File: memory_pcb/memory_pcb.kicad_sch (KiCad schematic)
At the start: 48 parts, among them J1 Conn_01x10, P1 AFC01-S10FCC-00, U1 AP3602AKTR-G1 SETUPUP, U10 DMG3415U, U11 SS54_C22452, U12 TYPE-C-31-M-12, U2 ESP32-S3-WROOM-1(N16R8), U4 TS-1088-AR02016, U5 TS-1088-AR02016, U6 MAX17048G+T10 FUEL GAUGE, U7 MCP73831T-2ACI/OT Charger, U8 S2B-PH-SM4-TB(LF)(SN)JST-PH C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, U9 AP2112K-3_3TRG1 Regulator

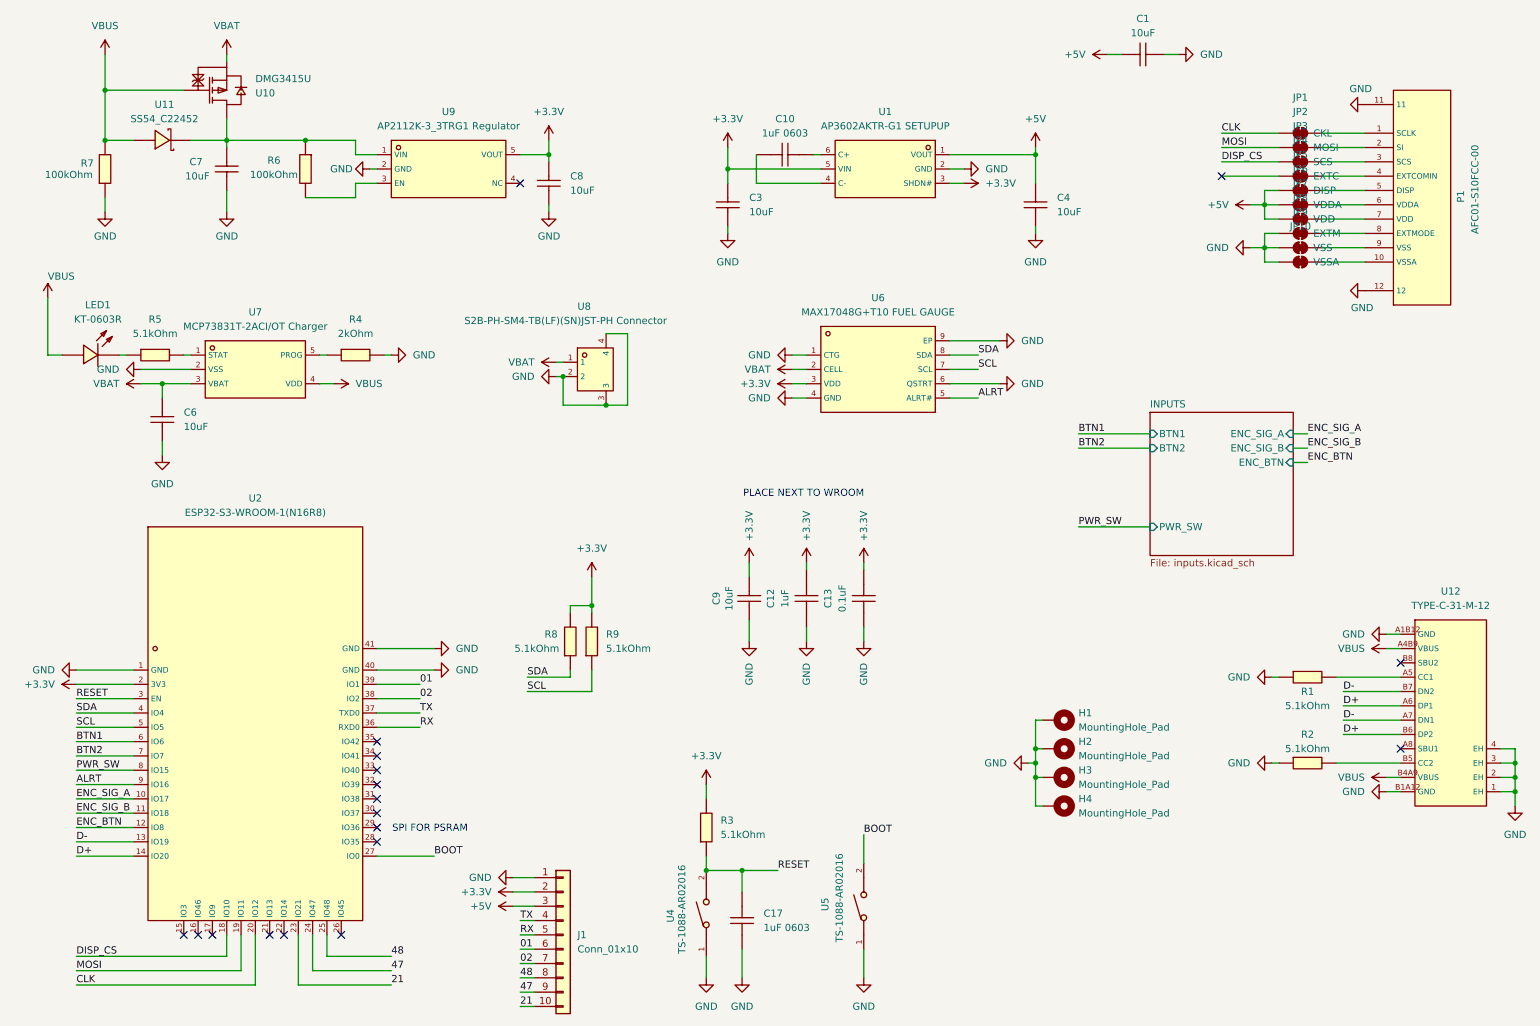
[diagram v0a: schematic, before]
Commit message: looks rdy
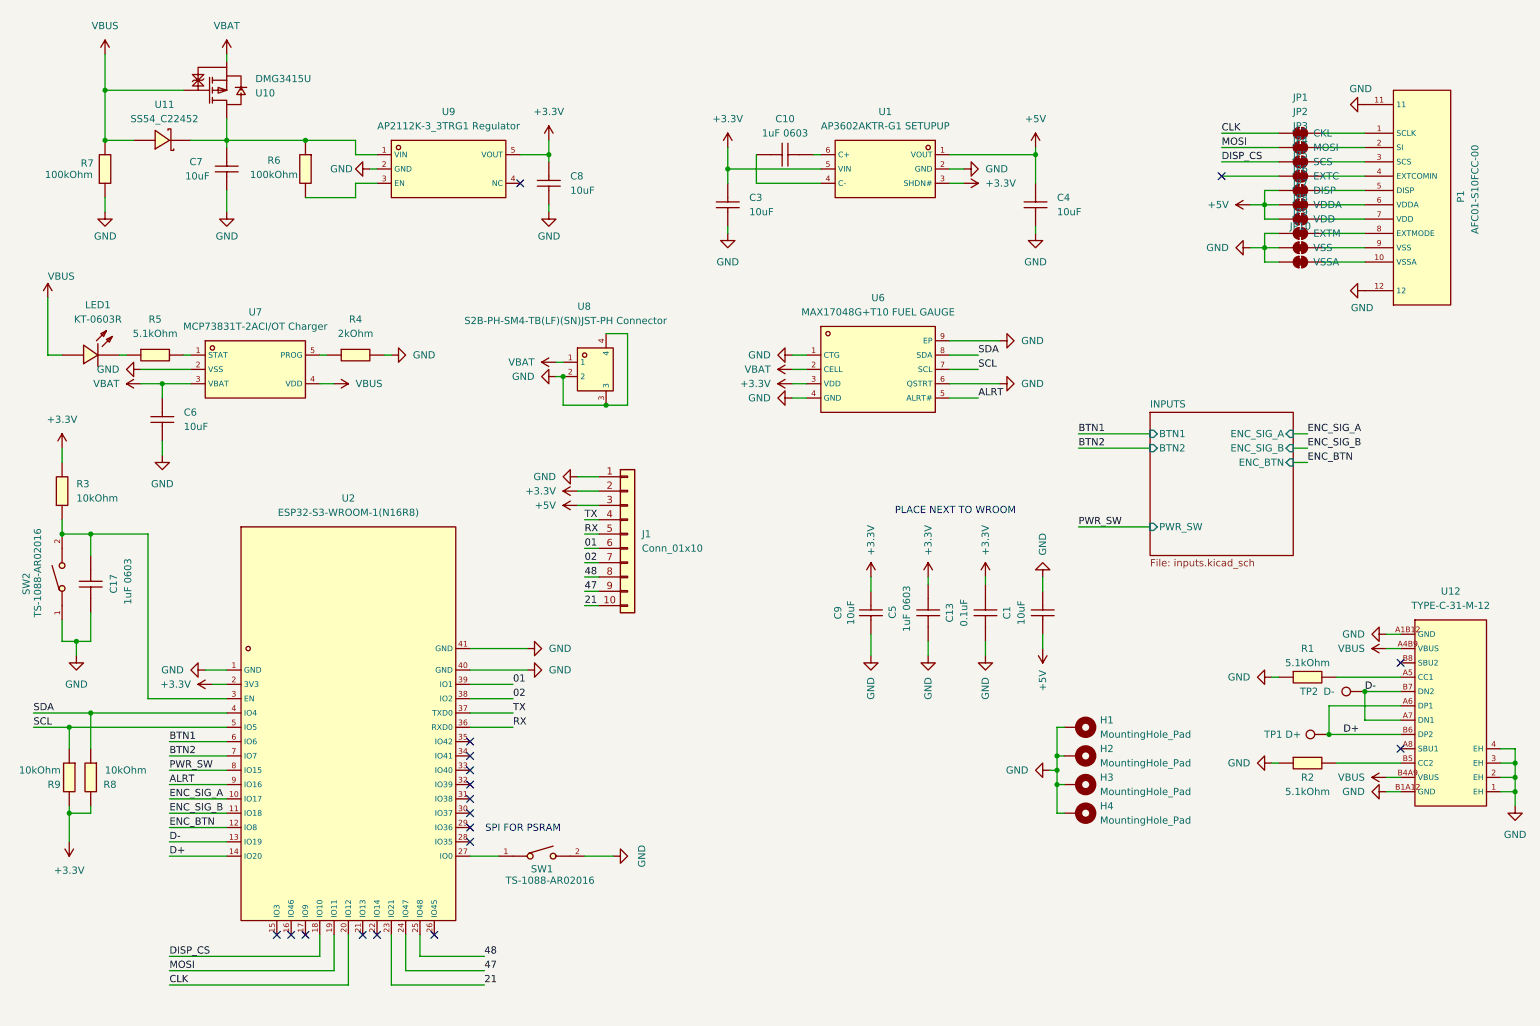
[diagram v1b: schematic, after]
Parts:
- removed C12: 1uF, new_lib_footprint:C1206, symbol new_lib_symbol:CL31B105KBHNNNE
- added C5: 1uF 0603, new_lib_footprint:C0603, symbol new_lib_symbol:CL10A105KB8NNNC
- added TP1: D+, TestPoint:TestPoint_Pad_D1.0mm, symbol Connector:TestPoint
- added TP2: D-, TestPoint:TestPoint_Pad_D1.0mm, symbol Connector:TestPoint
- R3, R8, R9: value 5.1kOhm -> 10kOhm; LCSC C23186 -> C25804
- renumbered U5 to SW1, U4 to SW2
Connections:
- net +3.3V: now also C5.1
- net D+: now also TP1.1
- net D-: now also TP2.1
- net GND: now also SW1.2, C5.2; no longer SW1.1
- net BOOT: no longer names the net of U2.27 (IO0)
- net BOOT: now also SW1.1; no longer SW1.2
- net RESET: no longer names the net of C17.2, R3.1, SW2.2, U2.3 (EN)
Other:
- moved on the sheet: C1, C13, C17, C9, H1, H2, H3, H4, J1, R3, R8, R9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
